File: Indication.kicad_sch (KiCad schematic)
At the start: 13 parts

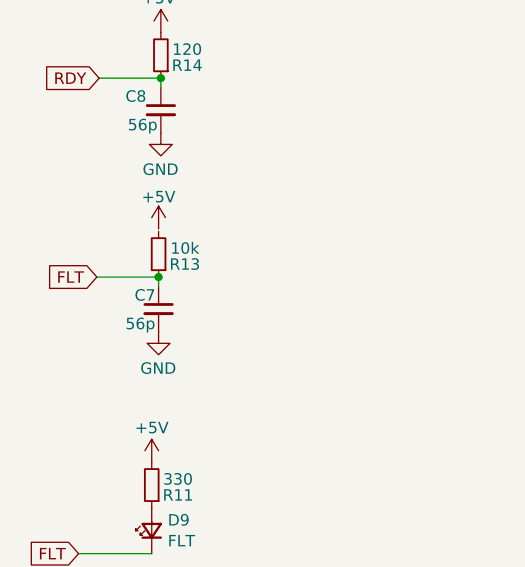
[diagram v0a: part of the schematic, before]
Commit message: Развел все дорожки
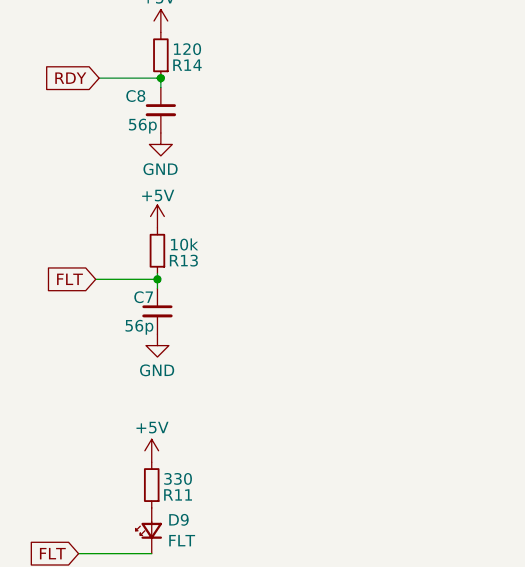
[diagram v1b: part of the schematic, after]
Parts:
- D6: footprint (none) -> Package_TO_SOT_SMD:SOT-23-5
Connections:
- net +5V: now also R13.2
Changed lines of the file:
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@@
-	)
-	(junction
-		(at 76.962 83.566)
-		(diameter 0)
-		(color 0 0 0 0)
 	)
 	(junction
@@
 		(color 0 0 0 0)
 	)
+	(junction
+		(at 76.835 83.82)
+		(diameter 0)
+		(color 0 0 0 0)
+	)
 	(no_connect
 		(at 221.996 95.758)
@@
 	(wire
 		(pts
+			(xy 76.835 83.185) (xy 76.835 83.82)
+		)
+		(stroke
+			(width 0)
+			(type default)
+		)
+	)
+	(wire
+		(pts
 			(xy 242.57 105.41) (xy 242.57 106.426)
 		)
@@
 	(wire
 		(pts
-			(xy 70.104 83.566) (xy 76.962 83.566)
+			(xy 69.977 83.82) (xy 76.835 83.82)
 		)
 		(stroke
@@
 	(wire
 		(pts
-			(xy 76.962 84.582) (xy 76.962 83.566)
+			(xy 76.835 84.836) (xy 76.835 83.82)
 		)
 		(stroke
@@
 	(global_label "FLT"
 		(shape input)
-		(at 70.104 83.566 180)
+		(at 69.977 83.82 180)
 		(fields_autoplaced yes)
 		(effects
@@
 		)
 		(property "Intersheetrefs" "${INTERSHEET_REFS}"
-			(at 64.0345 83.566 0)
+			(at 63.9075 83.82 0)
 			(effects
 				(font
@@
 	(symbol
 		(lib_id "power:+5V")
-		(at 76.962 78.232 0)
+		(at 76.835 78.105 0)
 		(unit 1)
 		(exclude_from_sim no)
@@
 		(dnp no)
 		(property "Reference" "#PWR017"
-			(at 76.962 82.042 0)
+			(at 76.835 81.915 0)
 			(effects
 				(font
@@
 		)
 		(property "Value" "+5V"
-			(at 76.962 74.676 0)
+			(at 76.835 74.549 0)
 			(effects
 				(font
@@
 		)
 		(property "Footprint" ""
-			(at 76.962 78.232 0)
+			(at 76.835 78.105 0)
 			(effects
 				(font
@@
 		)
 		(property "Datasheet" ""
-			(at 76.962 78.232 0)
+			(at 76.835 78.105 0)
 			(effects
 				(font
@@
 		)
 		(property "Description" "Power symbol creates a global label with name \"+5V\""
-			(at 76.962 78.232 0)
+			(at 76.835 78.105 0)
 			(effects
 				(font
@@
 			)
 		)
-		(property "Footprint" ""
+		(property "Footprint" "Package_TO_SOT_SMD:SOT-23-5"
 			(at 177.292 99.06 0)
 			(effects
@@
 	(symbol
 		(lib_id "power:GND")
-		(at 76.962 89.662 0)
+		(at 76.835 89.916 0)
 		(unit 1)
 		(exclude_from_sim no)
@@
 		(dnp no)
 		(property "Reference" "#PWR018"
-			(at 76.962 96.012 0)
+			(at 76.835 96.266 0)
 			(effects
 				(font
@@
 		)
 		(property "Value" "GND"
-			(at 74.93 93.726 0)
+			(at 74.803 93.98 0)
 			(effects
 				(font
@@
 		)
 		(property "Footprint" ""
-			(at 76.962 89.662 0)
+			(at 76.835 89.916 0)
 			(effects
 				(font
@@
 		)
 		(property "Datasheet" ""
-			(at 76.962 89.662 0)
+			(at 76.835 89.916 0)
 			(effects
 				(font
@@
 		)
 		(property "Description" ""
-			(at 76.962 89.662 0)
+			(at 76.835 89.916 0)
 			(effects
 				(font
@@
 	(symbol
 		(lib_id "Device:C_Small")
-		(at 76.962 87.122 0)
+		(at 76.835 87.376 0)
 		(unit 1)
 		(exclude_from_sim no)
@@
 		(dnp no)
 		(property "Reference" "C7"
-			(at 74.295 85.598 0)
+			(at 74.168 85.852 0)
 			(effects
 				(font
@@
 		)
 		(property "Value" "56p"
-			(at 73.279 88.773 0)
+			(at 73.152 89.027 0)
 			(effects
 				(font
@@
 		)
 		(property "Footprint" "Capacitor_SMD:C_0805_2012Metric_Pad1.18x1.45mm_HandSolder"
-			(at 76.962 87.122 0)
+			(at 76.835 87.376 0)
 			(effects
 				(font
@@
 		)
 		(property "Datasheet" "~"
-			(at 76.962 87.122 0)
+			(at 76.835 87.376 0)
 			(effects
 				(font
@@
 		)
 		(property "Description" ""
-			(at 76.962 87.122 0)
+			(at 76.835 87.376 0)
 			(effects
 				(font
@@
 	(symbol
 		(lib_id "Device:R_Small")
-		(at 76.962 81.026 180)
+		(at 76.835 80.645 180)
 		(unit 1)
 		(exclude_from_sim no)
@@
 		(dnp no)
 		(property "Reference" "R13"
-			(at 79.883 82.169 0)
+			(at 79.756 81.788 0)
 			(effects
 				(font
@@
 		)
 		(property "Value" "10k"
-			(at 79.883 80.391 0)
+			(at 79.756 80.01 0)
 			(effects
 				(font
@@
 		)
 		(property "Footprint" "Resistor_SMD:R_0805_2012Metric_Pad1.20x1.40mm_HandSolder"
-			(at 76.962 81.026 0)
+			(at 76.835 80.645 0)
 			(effects
 				(font
@@
 		)
 		(property "Datasheet" "~"
-			(at 76.962 81.026 0)
+			(at 76.835 80.645 0)
 			(effects
 				(font
@@
 		)
 		(property "Description" ""
-			(at 76.962 81.026 0)
-			(effects
-				(font
+			(at 76.835 80.645 0)
+			(effects
+				(font
